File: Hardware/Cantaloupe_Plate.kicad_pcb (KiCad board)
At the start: 2 copper layers, 142.1 x 117 mm, 36 parts, among them SW1 MX, SW10 MX, SW11 MX, SW12 MX, SW13 MX, SW14 MX, SW15 MX, SW16 MX, SW17 MX, SW18 MX, SW19 MX, SW2 MX, SW20 MX, SW21 MX, SW22 MX, SW23 MX, SW24 MX, SW25 MX, SW26 MX, SW27 MX, SW28 MX, SW29 MX, SW3 MX, SW30 MX, SW31 MX, SW4 MX, SW5 MX, SW6 MX, SW7 MX, SW8 MX, SW9 MX

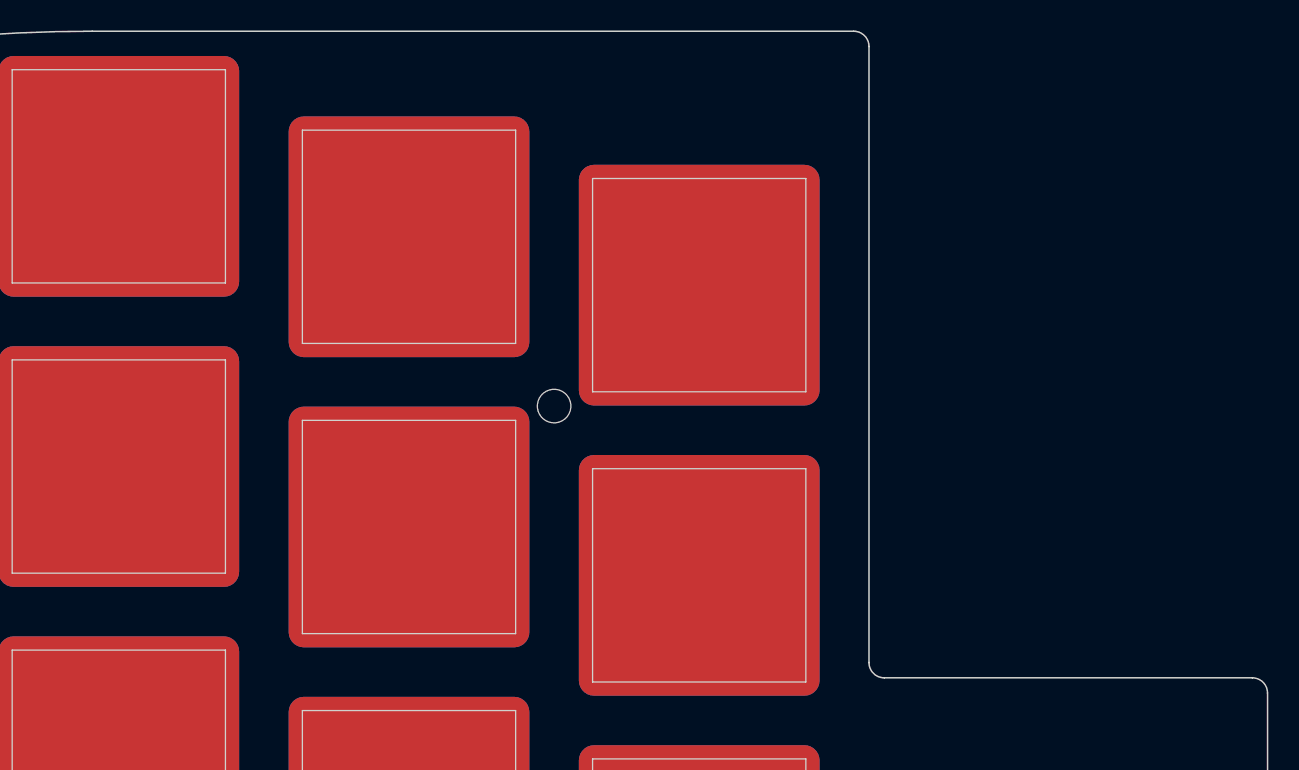
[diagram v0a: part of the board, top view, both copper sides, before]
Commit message: Updated to V1.2
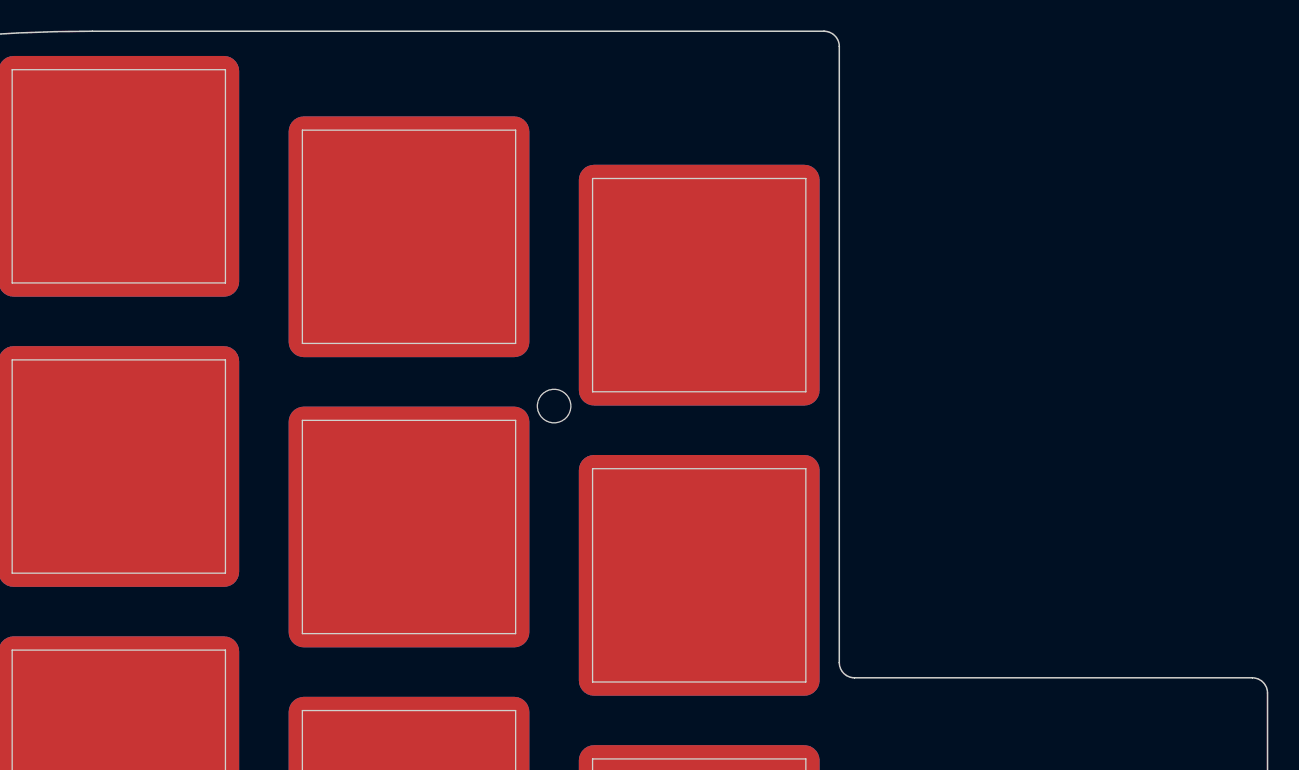
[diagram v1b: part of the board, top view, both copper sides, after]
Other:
- outline, holes or cut-outs redrawn
